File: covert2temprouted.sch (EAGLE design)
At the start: 44 parts, among them J1 B2B-PH-K-S(LF)(SN), U1 STM32G081RBT6

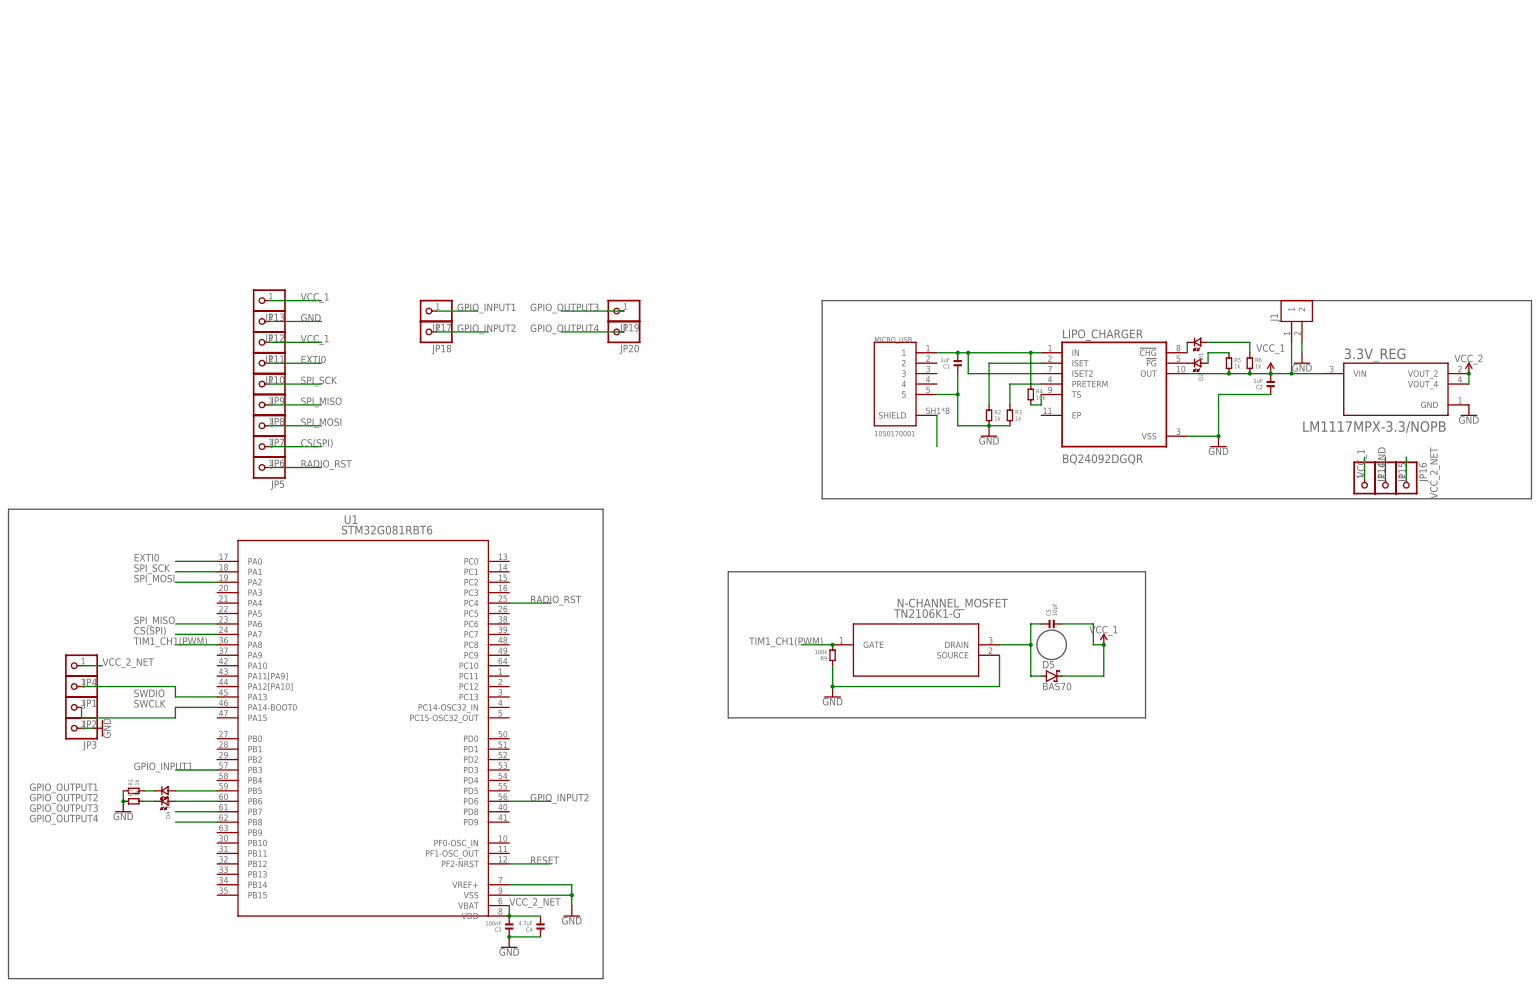
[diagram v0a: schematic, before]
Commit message: clean up
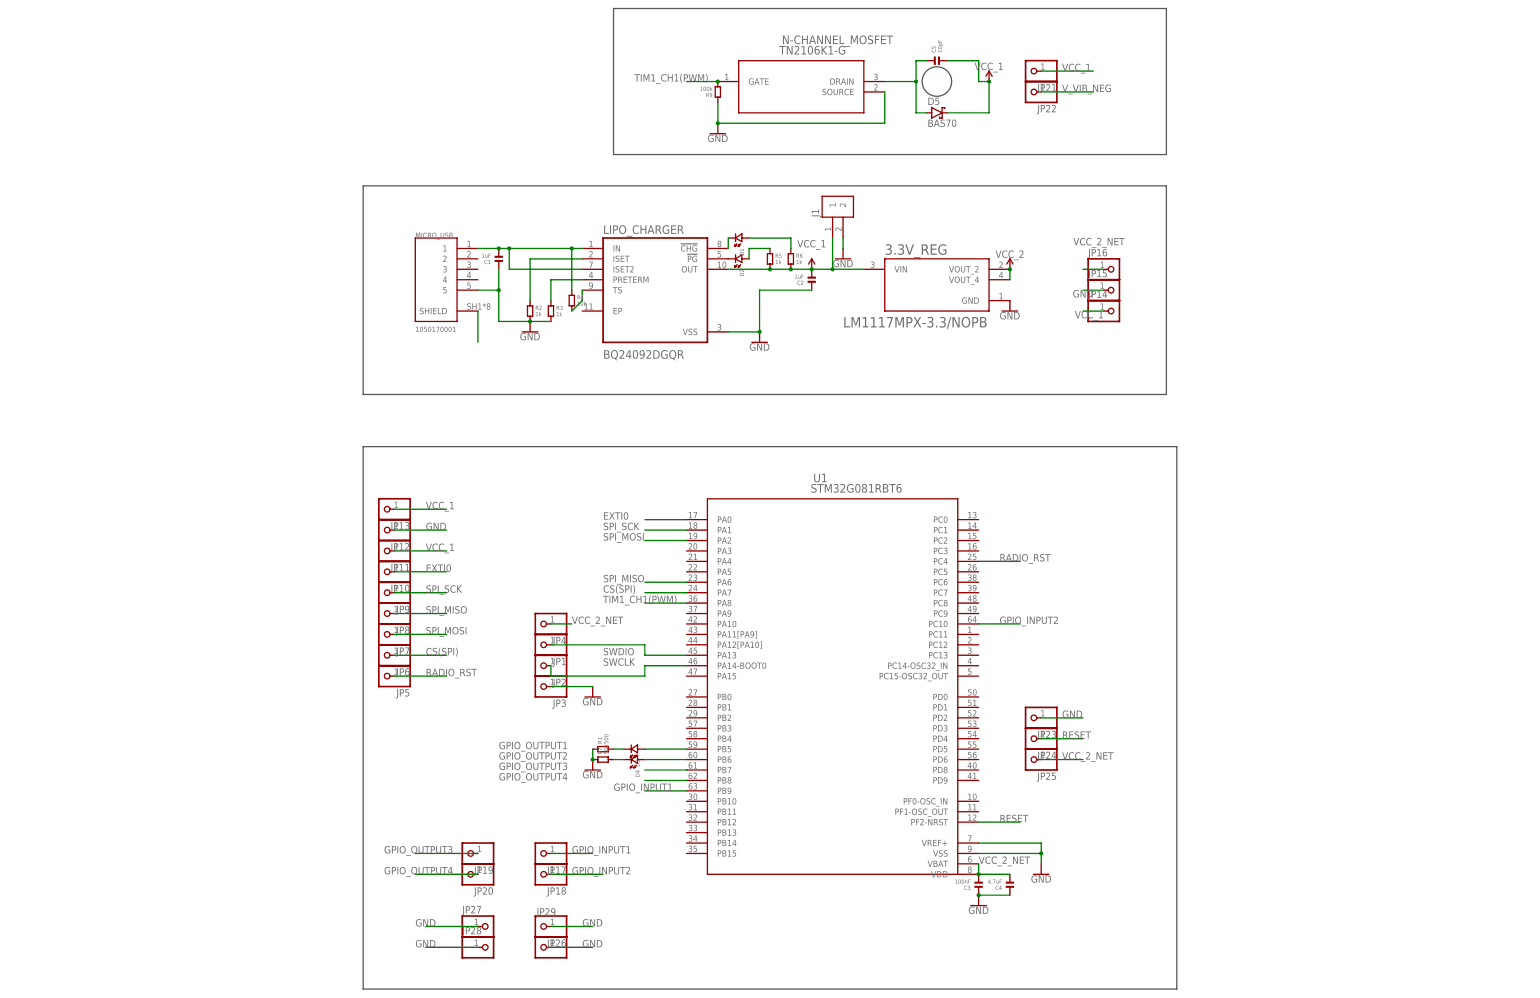
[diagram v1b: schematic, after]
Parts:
- added JP21, JP22, JP23, JP24, JP25, JP26, JP27, JP28, JP29: (no value), pinhead:PINHD-1X1
- R1, R7: value 1k -> 500
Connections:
- net GND: now also JP23.1, JP26.1, JP27.1, JP28.1, JP29.1
- net GPIO_INPUT1: now also U1.PB9; no longer U1.PB3
- net GPIO_INPUT2: now also U1.PC10; no longer U1.PD6
- net RESET: now also JP24.1
- net VCC_1: now also JP21.1
- net VCC_2_NET: now also JP25.1
- net V_VIB_NEG: now also JP22.1
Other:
- moved on the sheet: 3.3V_REG, C1, C2, C3, C4, C5, D1, D2, D3, D4, D5, J1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
